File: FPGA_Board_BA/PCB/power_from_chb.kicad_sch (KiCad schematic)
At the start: 5 parts, among them J4 Plug_Terminal_2x12pin, J5 Plug_Terminal_2x12pin, J6 Plug_Terminal_2x12pin, J7 Plug_Terminal_2x12pin, J8 Box_Header_6pin

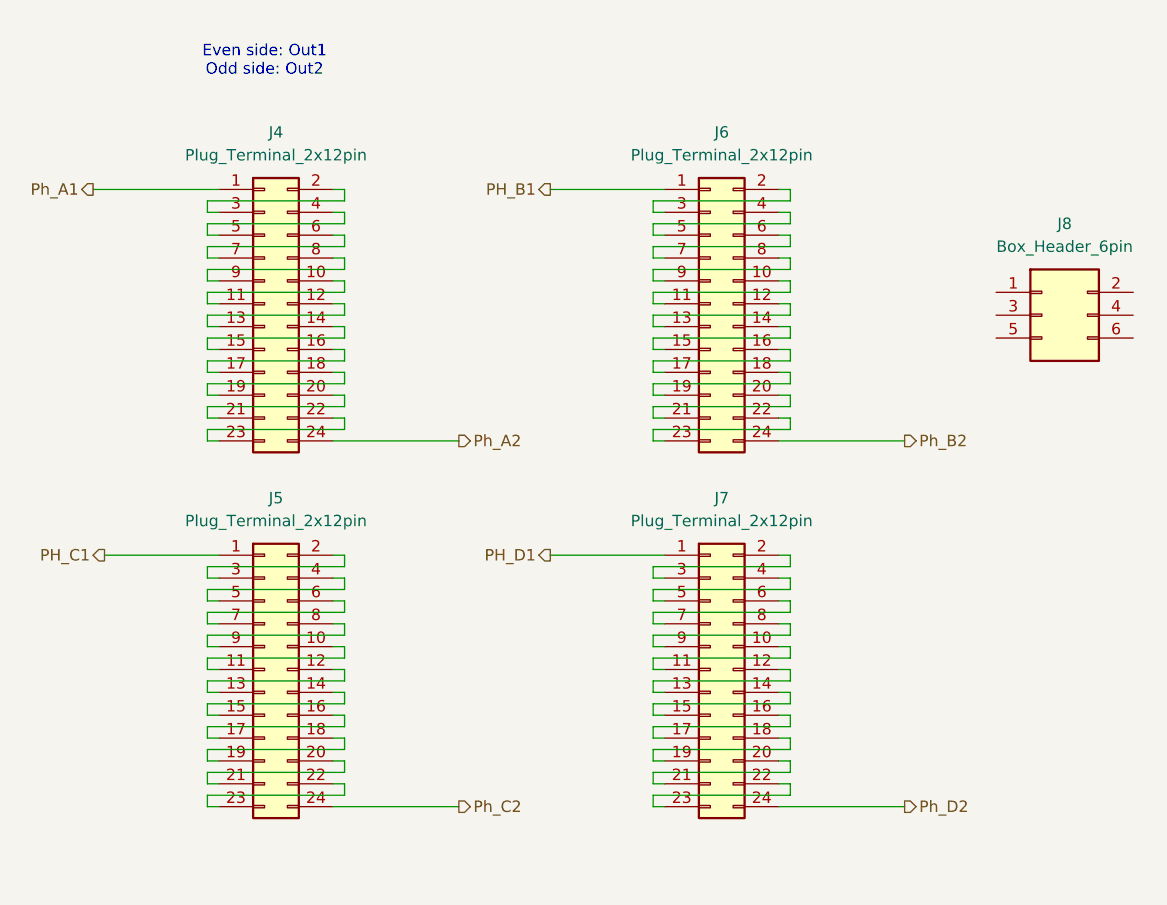
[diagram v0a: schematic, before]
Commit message: 22.11
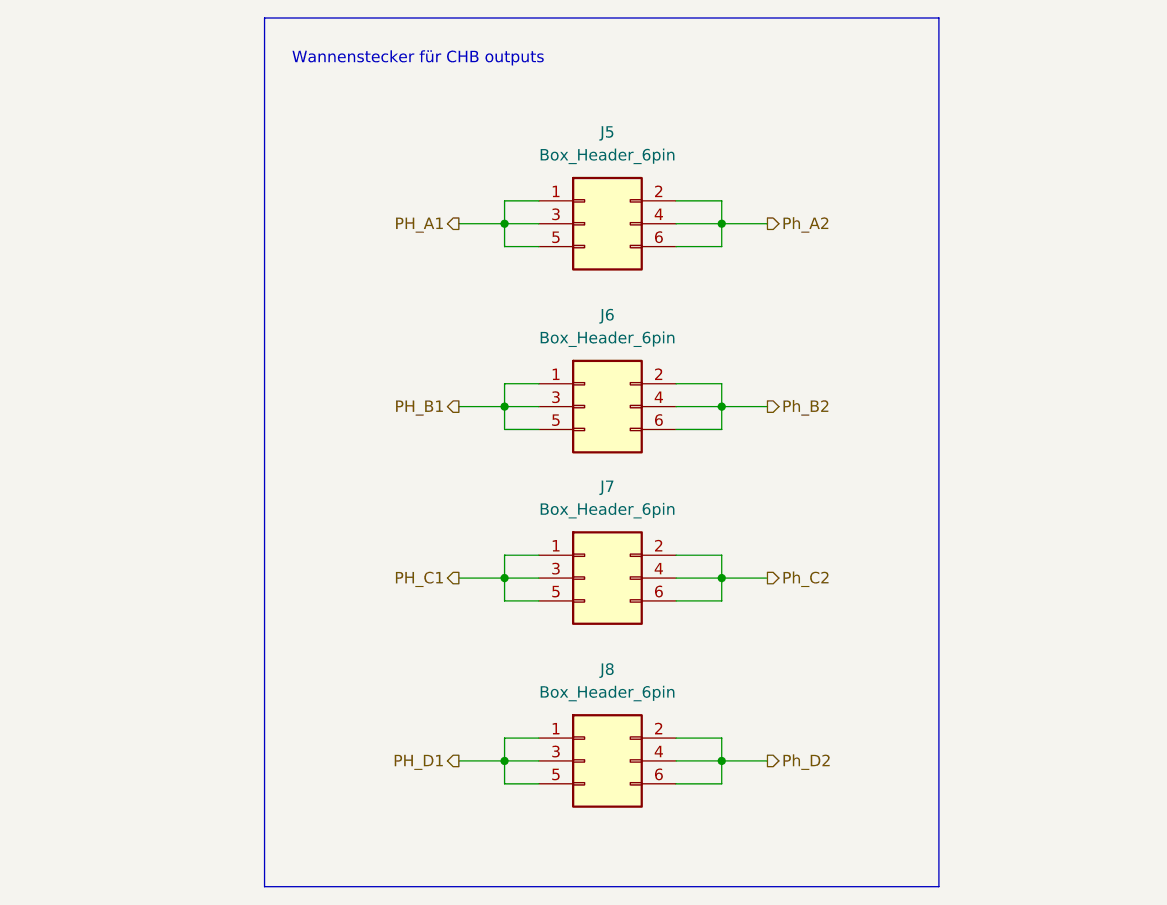
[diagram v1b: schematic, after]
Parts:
- removed J4, J5, J6, J7: Plug_Terminal_2x12pin, MYLIB_Misc:DMCV 1,5_12-G1F-3,5-LR P20THR, symbol MYLIB_Misc:Plug_Terminal_2x12pin
- added J6, J7, J8: Box_Header_6pin, Connector_IDC:IDC-Header_2x03_P2.54mm_Vertical, symbol MYLIB_Misc:Box_Header_6pin
- renumbered J8 to J5
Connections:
- net PH_B1: now also J6.1 (Pin_1), J6.3 (Pin_3), J6.5 (Pin_5)
- net PH_C1: now also J7.1 (Pin_1), J7.3 (Pin_3), J7.5 (Pin_5)
- net PH_D1: now also J8.1 (Pin_1), J8.3 (Pin_3), J8.5 (Pin_5)
- net Ph_A2: now also J5.2 (Pin_2), J5.4 (Pin_4), J5.6 (Pin_6)
- net Ph_B2: now also J6.2 (Pin_2), J6.4 (Pin_4), J6.6 (Pin_6)
- net Ph_C2: now also J7.2 (Pin_2), J7.4 (Pin_4), J7.6 (Pin_6)
- net Ph_D2: now also J8.2 (Pin_2), J8.4 (Pin_4), J8.6 (Pin_6)
- net PH_A1: now reaches J5.1 (Pin_1)
- net PH_A1: now also J5.3 (Pin_3), J5.5 (Pin_5)
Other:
- note added: "Wannenstecker für CHB outputs"
- note removed: "Even side: Out1 Odd side: Out2"
- moved on the sheet: J5
